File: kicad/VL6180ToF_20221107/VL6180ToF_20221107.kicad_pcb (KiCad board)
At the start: 2 copper layers, 50.8 x 50.8 mm, 17 parts, among them J1 Conn_01x07, Q1 SSM6N42FE, U1 Si91841, U2 VL6180X

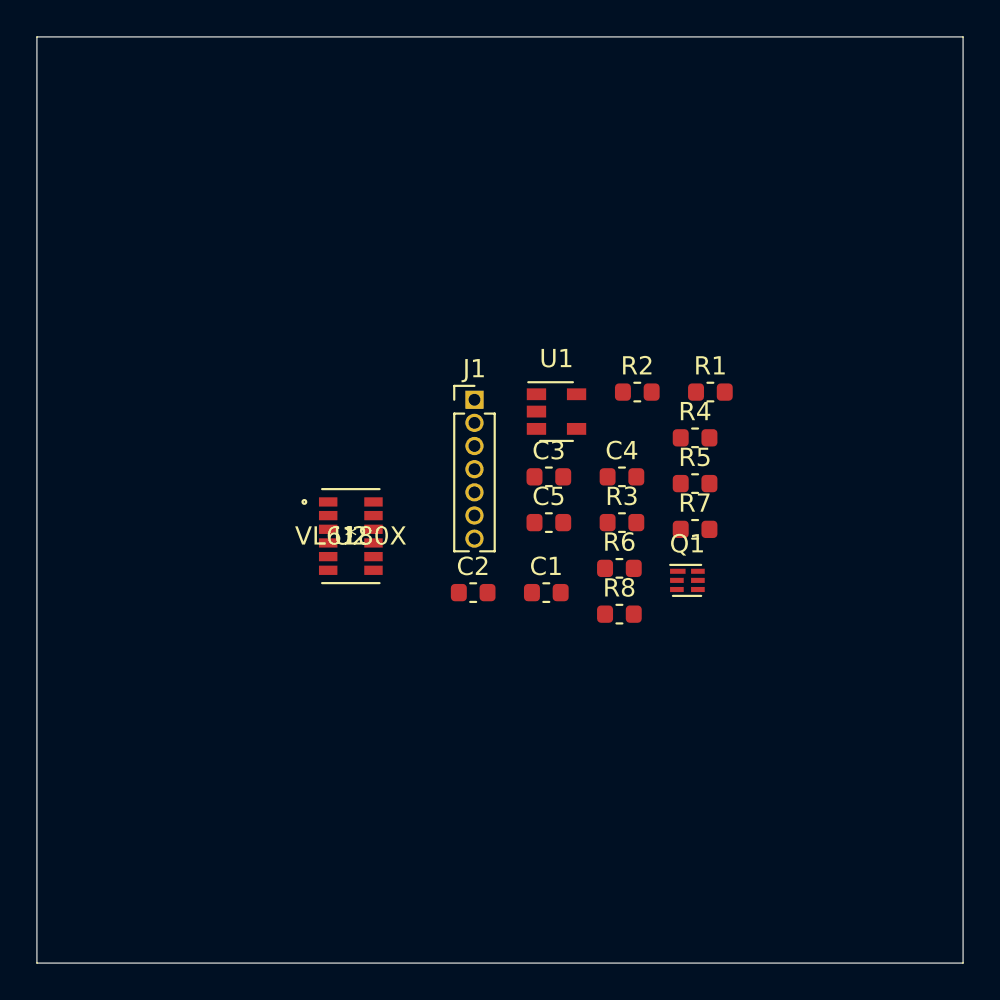
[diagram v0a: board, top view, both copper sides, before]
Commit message: kicad main+kick-drib
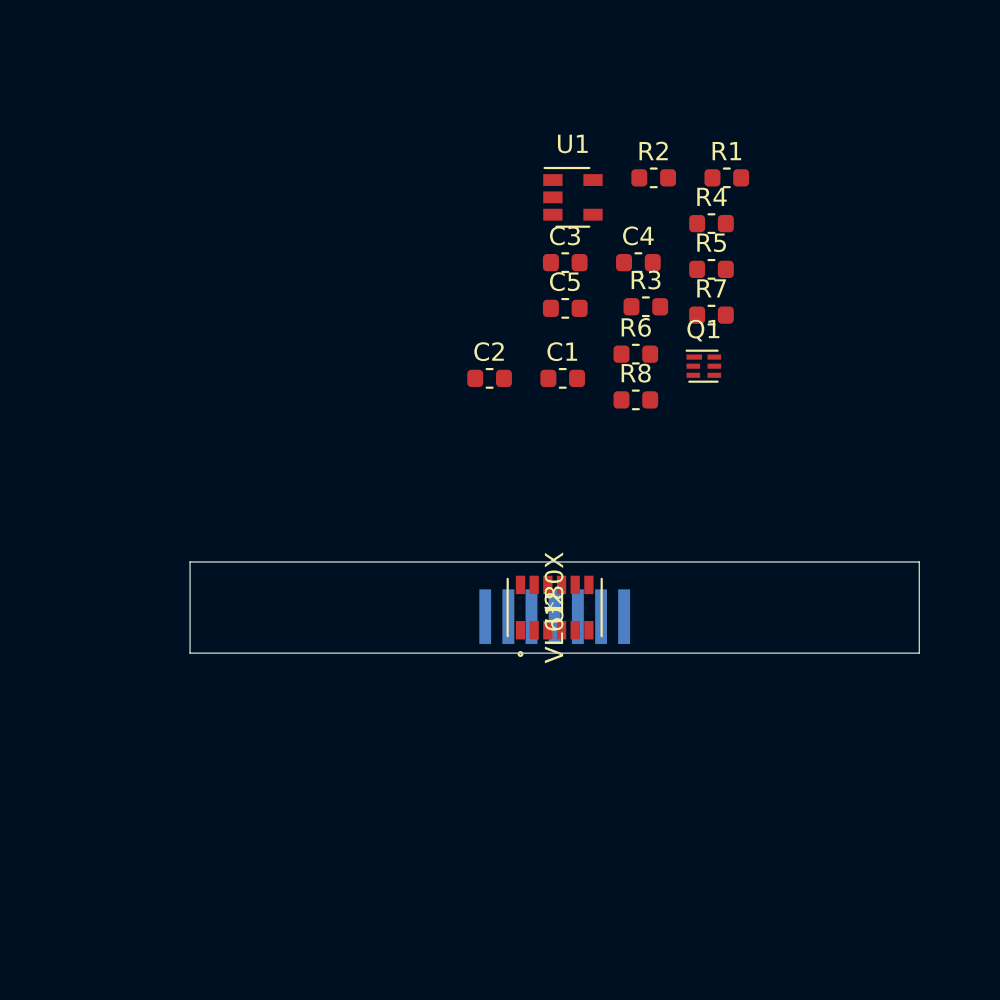
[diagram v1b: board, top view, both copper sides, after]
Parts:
- J1: footprint Connector_PinHeader_1.27mm:PinHeader_1x07_P1.27mm_Vertical -> 0.main.robot:Pin_1x07_P1.27mm_SMD; moved to B.Cu
- moved R3 11.9 mm to (135.0, 91.0)
- moved U2 11.8 mm to (130.0, 107.5), turned to 90 degrees
- moved C1 11.8 mm to (130.4, 94.9)
- moved C2 11.8 mm to (126.4, 94.9)
- moved C3 11.8 mm to (130.6, 88.6)
- moved C4 11.8 mm to (134.6, 88.6)
- moved C5 11.8 mm to (130.6, 91.1)
- moved Q1 11.8 mm to (138.2, 94.3)
- moved R1 11.8 mm to (139.4, 83.9)
- moved R2 11.8 mm to (135.4, 83.9)
- moved R4 11.8 mm to (138.6, 86.4)
- moved R5 11.8 mm to (138.6, 89.0)
- moved R7 11.8 mm to (138.6, 91.5)
- moved U1 11.8 mm to (131.0, 85.0)
- moved R6 11.8 mm to (134.4, 93.6)
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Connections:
- J1 pad 1: (no net) -> unconnected-(J1-Pad1)
- U2 pad 11: (no net) -> unconnected-(U2-Pad11)
- U2 pad 2: (no net) -> unconnected-(U2-Pad2)
- U2 pad 3: (no net) -> unconnected-(U2-Pad3)
- U2 pad 7: (no net) -> unconnected-(U2-Pad7)
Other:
- board size 50.8 x 50.8 mm -> 40 x 5 mm

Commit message: ToF
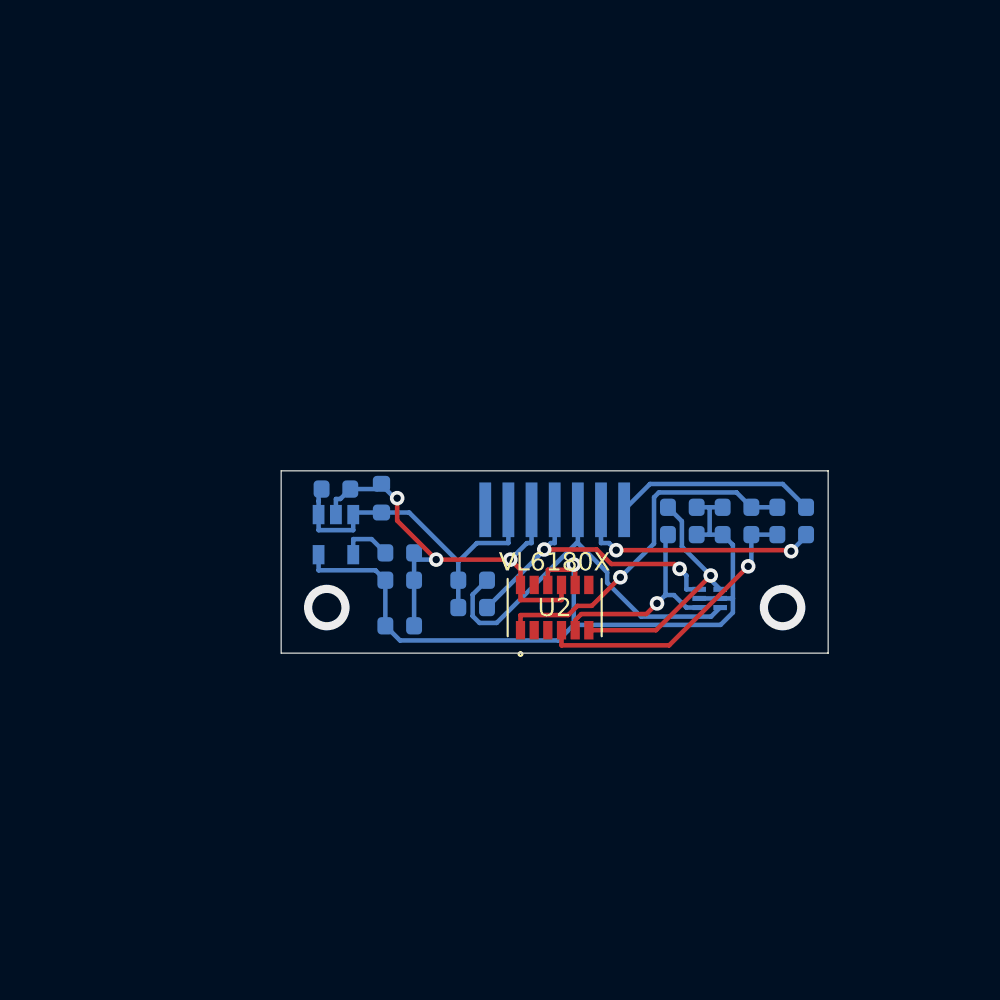
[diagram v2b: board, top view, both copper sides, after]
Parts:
- C1, C2, C3, C4, C5, Q1, R1, R2, R3, R4, R5, R6, R7, R8, U1: moved to B.Cu
- moved R1 26.1 mm to (125.5, 106.0)
- moved R2 25.6 mm to (125.5, 107.5)
- moved U1 22.6 mm to (118.0, 103.5), turned to -90 degrees
- moved C4 21.8 mm to (121.5, 106.0)
- moved C5 19.6 mm to (121.5, 108.5)
- moved C3 18.3 mm to (121.5, 104.5)
- moved R4 15.6 mm to (137.0, 102.0), turned to 180 degrees
- moved R5 14.6 mm to (140.0, 103.5)
- moved C1 13.8 mm to (118.0, 101.0)
- moved R7 12.8 mm to (143.0, 103.5)
- moved Q1 12.7 mm to (138.5, 107.0)
- moved R3 12.7 mm to (137.0, 103.5), turned to 180 degrees
- moved R8 10.4 mm to (143.0, 102.0)
- moved R6 10.1 mm to (140.0, 102.0)
- moved C2 8.85 mm to (120.5, 101.5), turned to 90 degrees
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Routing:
- net VDD: track 0.00 -> 44.7 mm, vias 0 -> 1
- net GND: track 0.00 -> 27.3 mm, vias 0 -> 3
- net Net-(J1-Pad5): track 0.00 -> 21.9 mm
- net Net-(R6-Pad2): track 0.00 -> 19.5 mm, vias 0 -> 1
- net VCC: track 0.00 -> 19.5 mm
- net Net-(J1-Pad4): track 0.00 -> 16.9 mm, vias 0 -> 2
- net Net-(R5-Pad2): track 0.00 -> 16.1 mm, vias 0 -> 1
- net Net-(J1-Pad6): track 0.00 -> 13.7 mm, vias 0 -> 2
- net Net-(Q1-Pad4): track 0.00 -> 13.6 mm, vias 0 -> 1
- net Net-(Q1-Pad1): track 0.00 -> 11.6 mm, vias 0 -> 1
- net Net-(J1-Pad7): track 0.00 -> 11.1 mm
- net Net-(C3-Pad1): track 0.00 -> 2.93 mm
- net (no net): vias 0 -> 2
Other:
- board size 40 x 5 mm -> 30 x 10 mm
